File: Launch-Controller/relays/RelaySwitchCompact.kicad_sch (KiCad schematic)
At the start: 11 parts, among them J1 350-10-105-00-001101, K1 1-1721150-0, U1 FOD817ASD, U2 FMMT634QTA

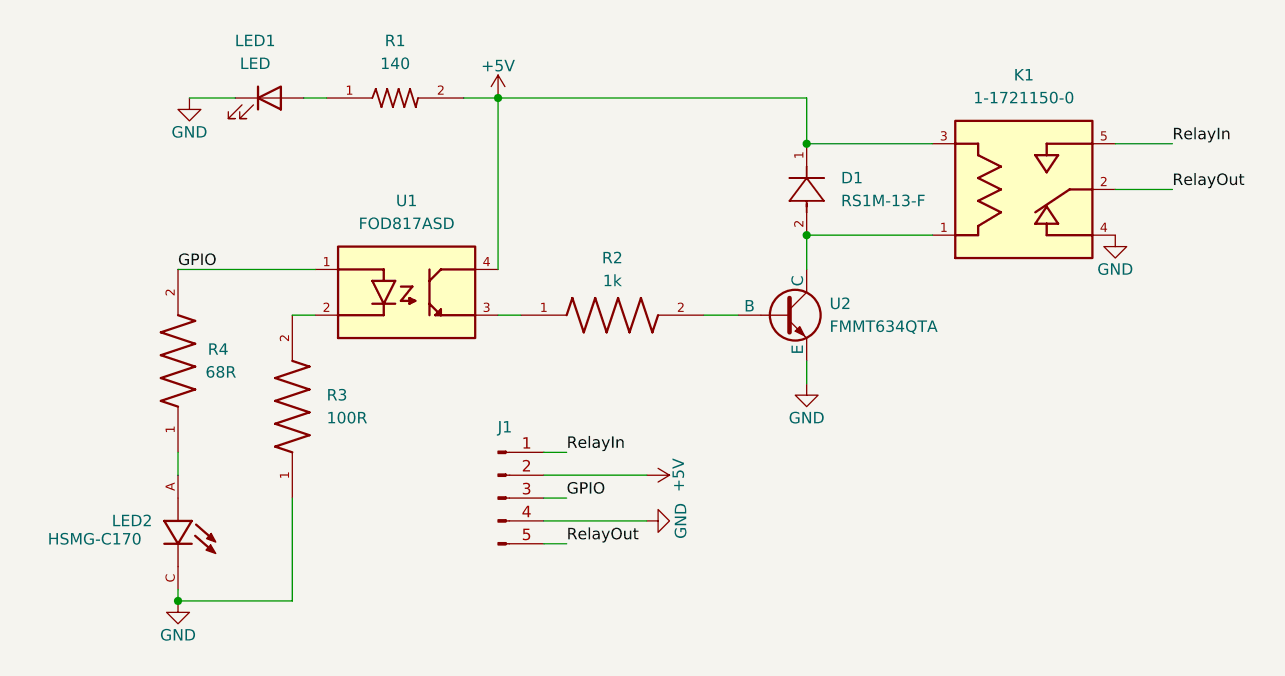
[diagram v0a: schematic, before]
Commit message: fab_files finalized
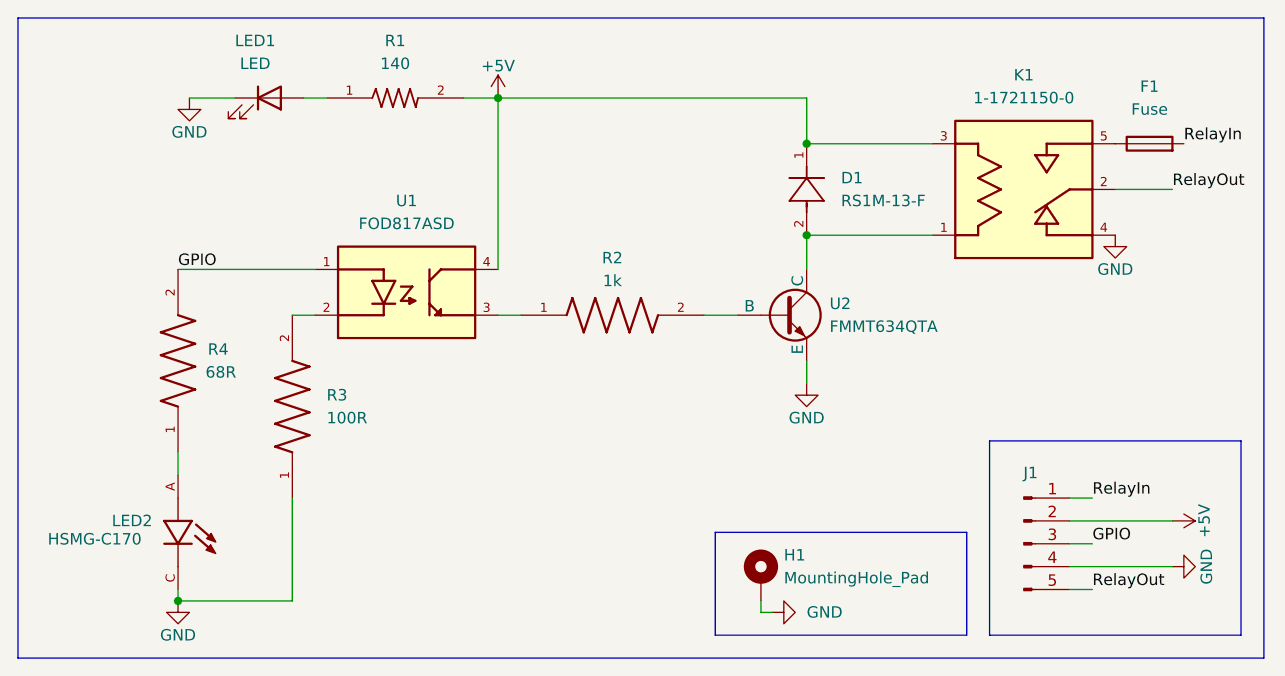
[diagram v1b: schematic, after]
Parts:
- added F1: Fuse, Diode_SMD:D_0402_1005Metric_Pad0.77x0.64mm_HandSolder, symbol Device:Fuse
- added H1: MountingHole_Pad, MountingHole:MountingHole_3.7mm_Pad, symbol Mechanical:MountingHole_Pad
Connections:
- net GND: now also H1.1
- net RelayIn: now also F1.2; no longer K1.5
- new net: F1.1, K1.5
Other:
- moved on the sheet: J1
